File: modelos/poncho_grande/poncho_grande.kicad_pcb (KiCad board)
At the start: 2 copper layers, 15 parts, among them K1 CONN_3, K2 CONN_3, P1 CONN_6, P10 CONN_4, P11 CONN_4, P12 CONN_5, P2 CONN_4, P3 CONN_5, P4 CONN_5, P5 CONN_4, P6 CONN_4, P7 CONN_5, P8 CONN_5, P9 CONN_6

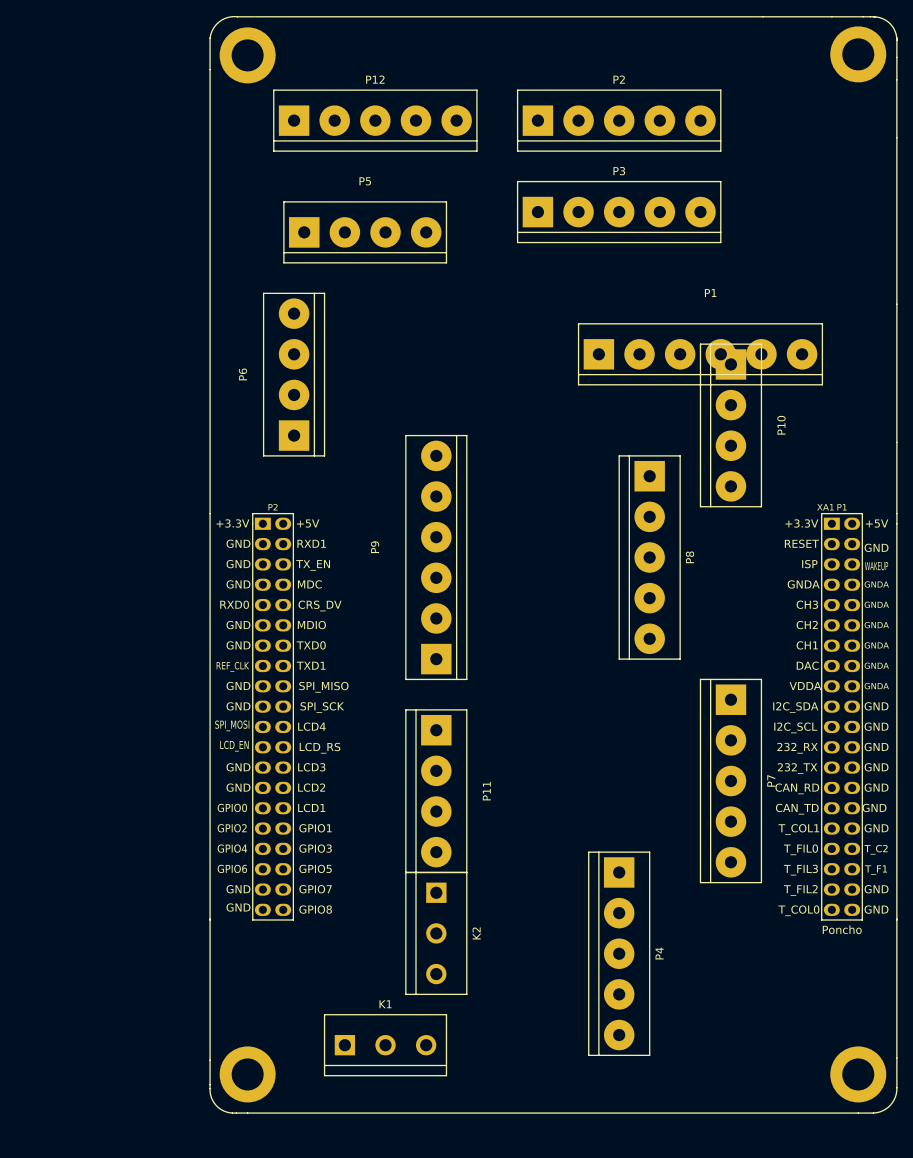
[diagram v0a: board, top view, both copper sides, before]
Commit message: * Mejoras y emprolijamiento en el esquemático y el PCB.
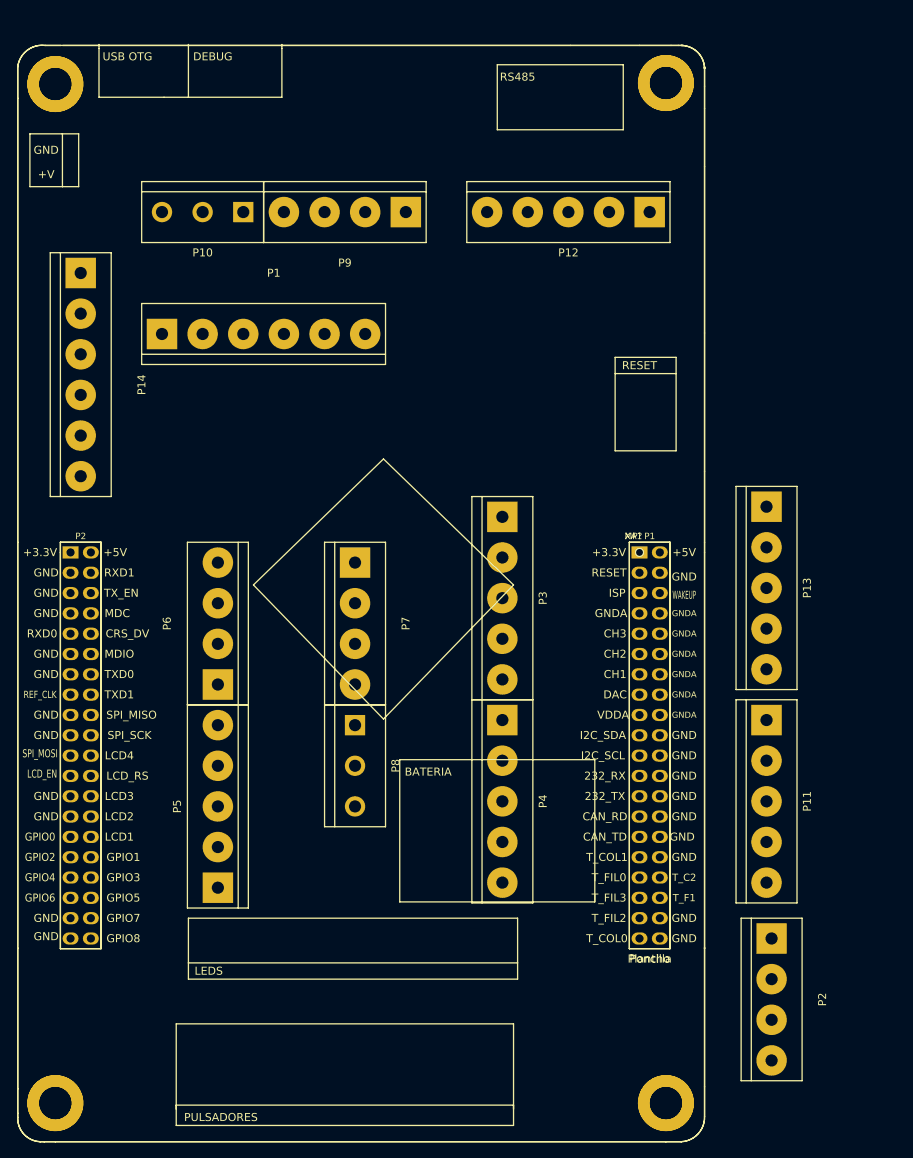
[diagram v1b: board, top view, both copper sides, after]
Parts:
- removed K1, K2: CONN_3, Connect:bornier3
- added MP?: Plantilla, mod:plantilla, F.Cu at (138.4, 92.1)
- added P13: CONN_5, mod:bornier5, F.Cu at (154.3, 96.5)
- added P14: CONN_6, mod:bornier6, F.Cu at (68.6, 69.8)
- P1: footprint Connect:bornier6 -> mod:bornier6
- P10: value CONN_4 -> CONN_3; footprint Connect:bornier4 -> mod:bornier3
- P11, P5: value CONN_4 -> CONN_5; footprint Connect:bornier4 -> mod:bornier5
- P12, P3, P4: footprint Connect:bornier5 -> mod:bornier5
- P2: footprint Connect:bornier5 -> mod:bornier4
- P6: footprint Connect:bornier4 -> mod:bornier4
- P7: value CONN_5 -> CONN_4; footprint Connect:bornier5 -> mod:bornier4
- P8: value CONN_5 -> CONN_3; footprint Connect:bornier5 -> mod:bornier3
- P9: value CONN_6 -> CONN_4; footprint Connect:bornier6 -> mod:bornier4
- moved P2 111.5 mm to (154.9, 148.0), turned to 270 degrees
- moved P5 74.1 mm to (85.7, 123.8), turned to 90 degrees
- moved P10 71.2 mm to (83.8, 49.5), turned to 180 degrees
- moved P1 54.7 mm to (91.4, 64.8)
- moved P7 50.9 mm to (102.9, 101.0)
- moved P3 50.4 mm to (121.3, 97.8), turned to 270 degrees
- moved P8 45.1 mm to (102.9, 118.7)
- moved P9 44.7 mm to (101.6, 49.5), turned to 180 degrees
- moved P11 41.3 mm to (154.3, 123.2)
- moved P6 32.5 mm to (85.7, 101.0)
- moved P12 26.7 mm to (129.5, 49.5), turned to 180 degrees
- moved XA1 24.3 mm to (138.4, 92.1)
- moved P4 24.0 mm to (121.3, 123.2)
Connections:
- P1 pad 1: +3V3 -> +3.3V
- P10 pad 1: /Circuito Principal/RESET -> /Circuito Principal/GPIO7
- P10 pad 2: /Circuito Principal/ISP -> /Circuito Principal/GPIO8
- P10 pad 3: /Circuito Principal/WAKEUP -> GND
- P11 pad 1: +5P -> +5V
- P11 pad 2: /Circuito Principal/GPIO4 -> +3.3V
- P11 pad 3: /Circuito Principal/GPIO5 -> /Circuito Principal/RD
- P11 pad 4: /Circuito Principal/GPIO6 -> /Circuito Principal/TD
- P12 pad 1: +5P -> +5V
- P12 pad 2: +3.3VP -> +3.3V
- P12 pad 3: /Circuito Principal/LCD1 -> /Circuito Principal/SDA
- P12 pad 4: /Circuito Principal/LCD2 -> /Conector del Poncho/SCL
- P12 pad 5: /Circuito Principal/LCD3 -> GND
- P2 pad 1: +5V -> /Circuito Principal/RESET
- P2 pad 2: +3V3 -> /Circuito Principal/ISP
- P2 pad 3: /Circuito Principal/RXD -> /Circuito Principal/WAKEUP
- P2 pad 4: /Circuito Principal/TXD -> GND
- P3 pad 2: +3V3 -> +3.3V
- P5 pad 1: /Circuito Principal/LCD4 -> +5VP
- P5 pad 2: /Circuito Principal/LCD_EN -> +3.3VP
- P5 pad 3: /Circuito Principal/RS -> /Circuito Principal/LCD1
- P5 pad 4: GND -> /Circuito Principal/LCD2
- P6 pad 1: +5P -> /Circuito Principal/LCD4
- P6 pad 2: +3.3VP -> /Circuito Principal/LCD_EN
- P6 pad 3: /Circuito Principal/GPIO0 -> /Circuito Principal/RS
- P6 pad 4: /Circuito Principal/GPIO0 -> GND
- P7 pad 1: +5V -> +5VP
- P7 pad 2: +3V3 -> +3.3VP
- P7 pad 3: /Circuito Principal/RD -> /Circuito Principal/GPIO0
- P7 pad 4: /Circuito Principal/TD -> /Circuito Principal/GPIO1
- P8 pad 1: +5V -> /Circuito Principal/GPIO2
- P8 pad 2: +3V3 -> /Circuito Principal/GPIO3
- P8 pad 3: /Circuito Principal/SDA -> GND
- P9 pad 1: +5P -> +5VP
- P9 pad 2: +3.3VP -> /Circuito Principal/GPIO4
- P9 pad 3: /Circuito Principal/spiCCK -> /Circuito Principal/GPIO5
- P9 pad 4: /Circuito Principal/MOSI -> /Circuito Principal/GPIO6
- XA1 pad 1: +3V3 -> +3.3V
- XA1 pad 17: +3.3VADC -> (no net)
- XA1 pad 42: +5P -> +5VP
- XA1 pad 44: /Circuito Principal/RXD1 -> (no net)
- XA1 pad 46: /Circuito Principal/TXEN -> (no net)
- XA1 pad 48: /Circuito Principal/MDC -> (no net)
- XA1 pad 49: /Circuito Principal/RXD0 -> (no net)
- XA1 pad 50: /Circuito Principal/CRS -> (no net)
- XA1 pad 52: /Circuito Principal/MDIO -> (no net)
- XA1 pad 54: /Circuito Principal/TXD0 -> (no net)
- XA1 pad 55: /Circuito Principal/RCLK -> (no net)
- XA1 pad 56: /Circuito Principal/TXD1 -> (no net)
- XA1 pad 72: /Circuito Principal/GPIO0 -> /Circuito Principal/GPIO1
